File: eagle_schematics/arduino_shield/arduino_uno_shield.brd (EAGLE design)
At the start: 53 x 57.1 mm, 20 parts

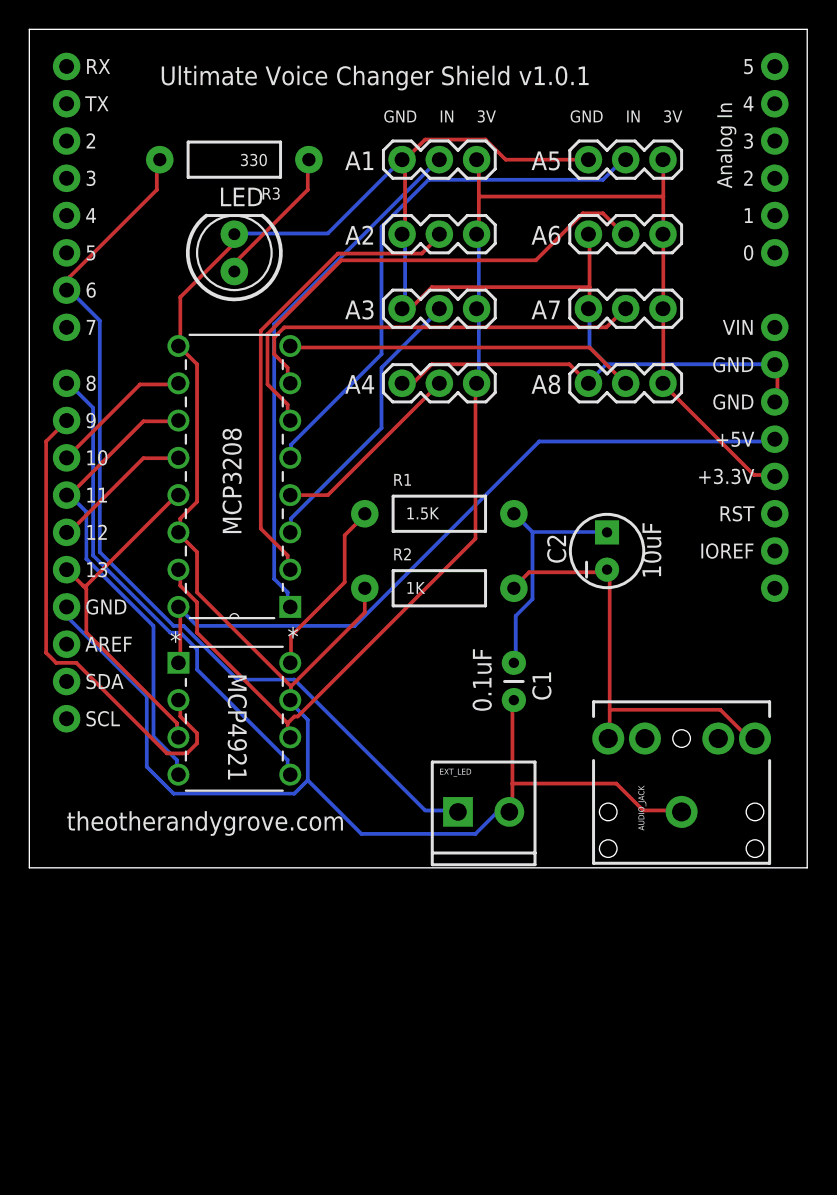
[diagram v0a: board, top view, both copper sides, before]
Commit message: save
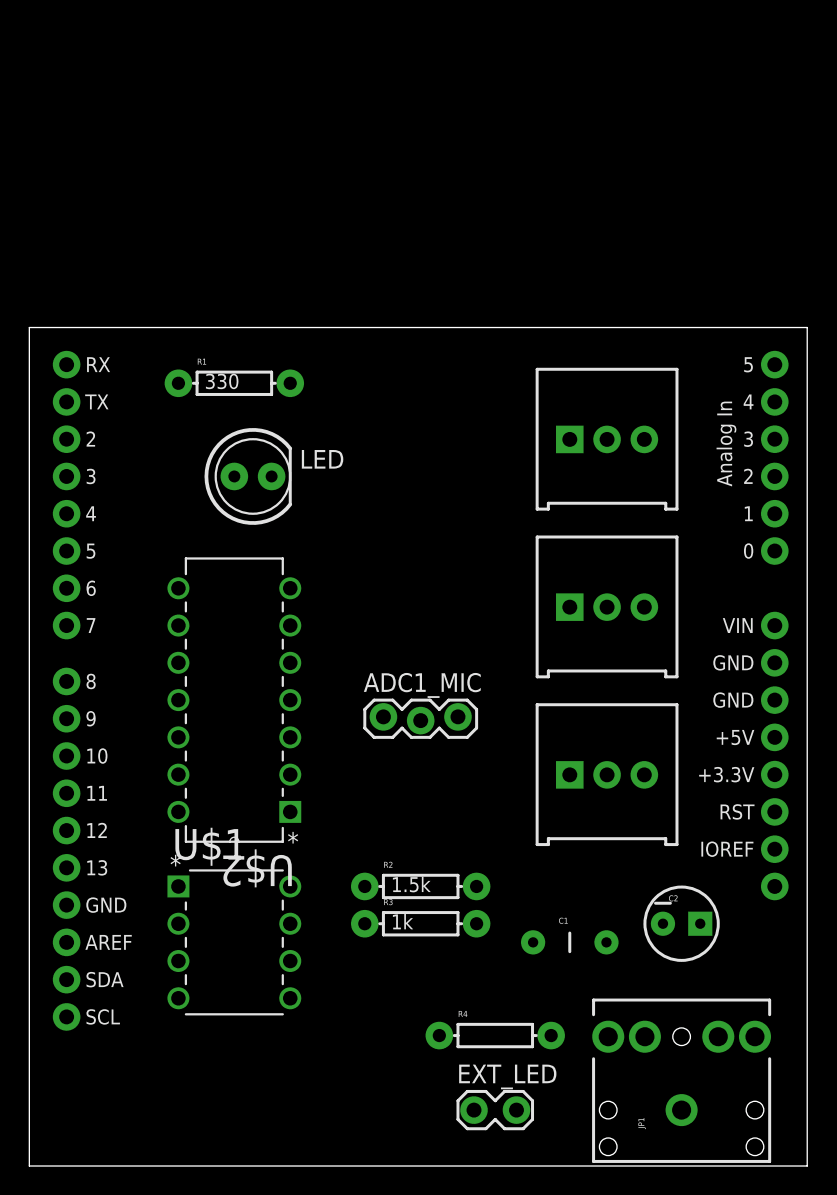
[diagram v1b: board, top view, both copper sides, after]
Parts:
- removed A1, A2, A3, A4, A5, A6, A7, A8: (no value), SparkFun-Connectors:1X03
- removed AUDIO_JACK: (no value), SparkFun-Connectors:AUDIO-JACK
- removed FRAME3: FRAME-LETTER, SparkFun-Aesthetics:CREATIVE_COMMONS
- removed MCP3208: MCP3208-CI/P, Microchip_By_element14_Batch_1:DIP254P762X432-16
- removed MCP4921: MCP4921-E/P, Microchip_By_element14_Batch_1:DIP254P762X432-8
- added ADC1_MIC: (no value), SparkFun-Connectors:1X03_LOCK
- added ADC2, ADC3, ADC4: TRIMPOT-PTH-KNOB, SparkFun-Electromechanical:3386U
- added JP1: (no value), SparkFun-Connectors:AUDIO-JACK
- added R4: (no value), SparkFun-Resistors:AXIAL-0.3
- added U$2: MCP3204-CI/P, Microchip_By_element14_Batch_1:DIP254P762X432-14
- added U1: ARDUINO_R3_SHIELD, SparkFun-Boards:UNO_R3_SHIELD
- C1: device SparkFun-Passives:CAP-PTH-SMALL -> SparkFun-Capacitors:CAP-PTH-5MM
- C2: device SparkFun-Passives:CPOL-RADIAL-10UF-25V -> SparkFun-Capacitors:CPOL-RADIAL-10UF-25V
- EXT_LED: value M023.5MM -> M02LOCK; device SparkFun-Connectors:SCREWTERMINAL-3.5MM-2 -> SparkFun-Connectors:1X02_LOCK
- R1: value 1.5K -> 330; device SparkFun-Passives:AXIAL-0.4 -> SparkFun-Resistors:AXIAL-0.3
- R2: value 1K -> 1.5k; device SparkFun-Passives:AXIAL-0.4 -> SparkFun-Resistors:AXIAL-0.3
- R3: value 330 -> 1k; device SparkFun-Passives:AXIAL-0.4 -> SparkFun-Resistors:AXIAL-0.3
- U$1: value ARDUINO_R3_SHIELD -> MCP4921-E/P; device SparkFun-Boards:UNO_R3_SHIELD -> Microchip_By_element14_Batch_1:DIP254P762X432-8
- moved R3 53.6 mm to (26.7, 16.5), turned to 0 degrees
- moved C2 25.9 mm to (44.5, 16.5), turned to 0 degrees
- moved EXT_LED 20.4 mm to (30.5, 3.81)
- moved R2 20.4 mm to (26.7, 19.1)
- moved U$1 19.9 mm to (17.8, 11.4)
- moved C1 19.4 mm to (36.8, 15.2), turned to 0 degrees
- moved R1 16.6 mm to (14.0, 53.3)
- moved LED 15.3 mm to (15.2, 47.0), turned to 0 degrees
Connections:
- removed net AUD: A1.2, MCP3208.1
- removed net N$10: LED.A, R3.P$1
- removed net N$11: MCP4921.5, U$1.D8
- removed net N$12: EXT_LED.1, R3.P$2, U$1.D6
- removed net N$14: A3.2, MCP3208.3
- removed net N$15: A4.2, MCP3208.4
- removed net N$16: A6.2, MCP3208.6
- removed net N$17: A7.2, MCP3208.7
- removed net N$18: A8.2, MCP3208.8
- removed net N$8: C1.1, C2.1, R1.P$2
- removed net N$9: AUDIO_JACK.RING, AUDIO_JACK.TIP, C2.2, R2.P$2
- removed net SPI_CLK: MCP3208.13, MCP4921.3, U$1.D13
- removed net SPI_MISO: MCP3208.12, U$1.D12
- removed net SPI_MOSI: MCP3208.11, MCP4921.4, U$1.D11
- new net ADC1: ADC1_MIC.1, U$2.1
- new net ADC2: ADC2.2, U$2.2
- new net ADC3: ADC3.2, U$2.3
- new net ADC4: ADC4.2, U$2.4
- new net LDAC: U$1.5, U1.D8
- new net LED: R1.P$1, R4.P$1, U1.D6
- new net MISO: U$2.10, U1.D12
- new net MOSI: U$1.4, U$2.9, U1.D11
- new net N$4: C2.2, JP1.RING, JP1.TIP, R3.P$2
- new net N$5: EXT_LED.1, R4.P$2
- new net SCK: U$1.3, U$2.11, U1.D13
- net 3.3V: now also ADC1_MIC.3, ADC2.1, ADC3.1, ADC4.1, U$1.6, U$2.13, U1.3.3V; no longer A1.3, A2.3, A3.3, A4.3, A5.3, A6.3, A7.3, A8.3, MCP3208.15, MCP4921.6, U$1.3.3V
- net 5V: now also U$1.1, U$2.14, U1.5V; no longer MCP3208.16, MCP4921.1, U$1.5V
- net CS_ADC: now also U$2.8, U1.D10; no longer MCP3208.10, U$1.D10
- net CS_DAC: now also U$1.2, U1.D9; no longer MCP4921.2, U$1.D9
- net GND: now also ADC1_MIC.2, ADC2.3, ADC3.3, ADC4.3, JP1.SLEEVE, R3.P$1, U$1.7, U$2.12, U$2.7, U1.GND@0; no longer A1.1, A2.1, A3.1, A4.1, A5.1, A6.1, A7.1, A8.1, AUDIO_JACK.SLEEVE, MCP3208.14, MCP3208.9, MCP4921.7, R2.P$1, U$1.GND@0, U$1.GND@1, U$1.GND@2
- net N$1: now also LED.A, R1.P$2; no longer A5.2, MCP3208.5
- net N$2: now also R2.P$1, U$1.8; no longer A2.2, MCP3208.2
- net N$3: now also C1.1, C2.1, R2.P$2; no longer MCP4921.8, R1.P$1
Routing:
- net GND: track 204.1 -> 0.00 mm
- net 3.3V: track 97.2 -> 0.00 mm
- net N$12: track 62.3 -> 0.00 mm
- net 5V: track 50.5 -> 0.00 mm
- net N$1: track 36.8 -> 0.00 mm
- net AUD: track 35.7 -> 0.00 mm
- net N$16: track 34.9 -> 0.00 mm
- net N$11: track 33.5 -> 0.00 mm
- net CS_DAC: track 33.3 -> 0.00 mm
- net N$2: track 32.1 -> 0.00 mm
- net SPI_MOSI: track 32.0 -> 0.00 mm
- net N$9: track 29.3 -> 0.00 mm
- net N$17: track 28.3 -> 0.00 mm
- net N$18: track 23.9 -> 0.00 mm
- net SPI_CLK: track 23.7 -> 0.00 mm
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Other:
- board text removed: "3V"
- board text removed: "GND"
- board text removed: "IN"
- board text removed: "Ultimate Voice Changer Shield v1.0.1"
- board text removed: "theotherandygrove.com"

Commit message: save
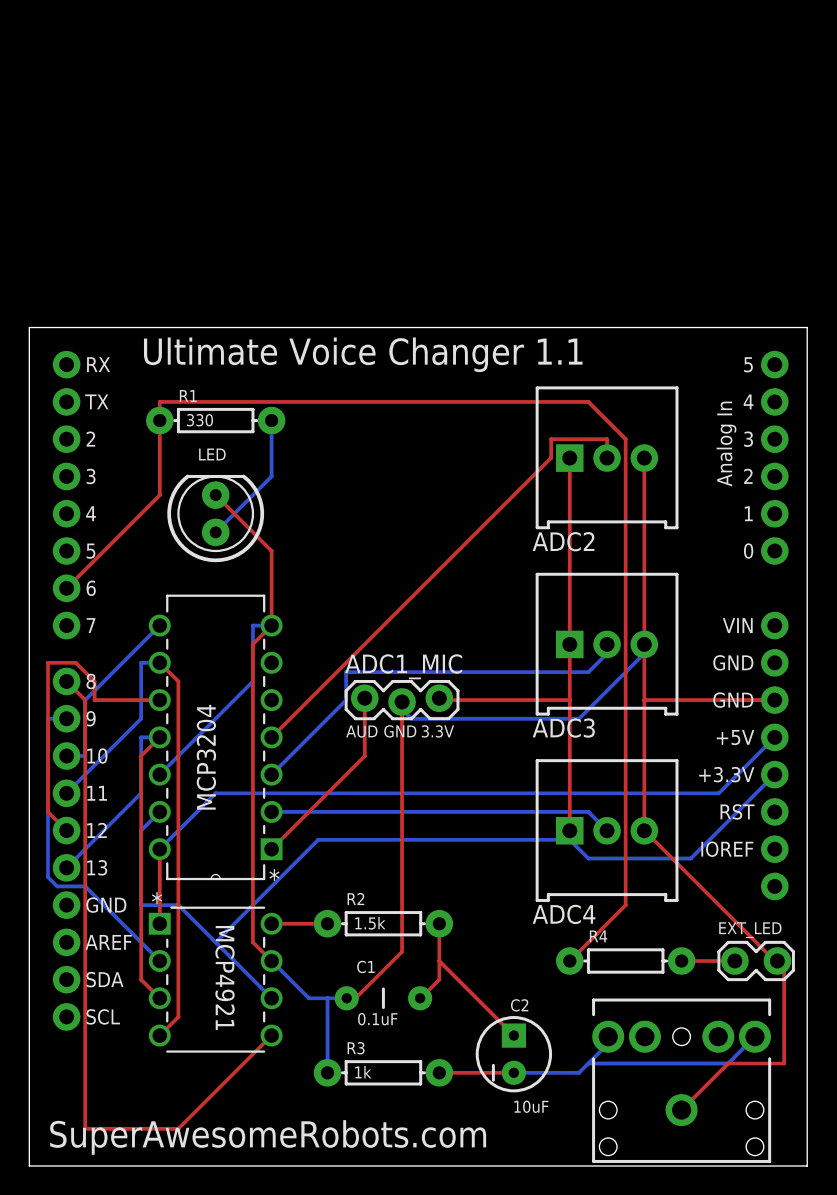
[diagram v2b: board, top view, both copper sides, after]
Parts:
- moved EXT_LED 20.5 mm to (48.3, 14.0)
- moved C2 14.5 mm to (33.0, 7.62), turned to 90 degrees
- moved C1 13.3 mm to (24.1, 11.4), turned to 180 degrees
- moved R3 10.5 mm to (24.1, 6.35)
- moved R4 10.2 mm to (40.6, 14.0)
- moved ADC2 3.81 mm to (39.4, 22.9)
- moved R2 3.59 mm to (24.1, 16.5)
- moved LED 3.59 mm to (12.7, 44.5), turned to 90 degrees
- moved R1 2.84 mm to (12.7, 50.8)
- moved U$1 2.84 mm to (16.5, 8.89)
- moved U$2 2.84 mm to (8.89, 36.8)
- moved ADC3 2.54 mm to (39.4, 35.6)
- moved ADC1_MIC 1.80 mm to (22.9, 31.8)
- moved ADC4 1.27 mm to (39.4, 48.3)
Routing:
- net GND: track 0.00 -> 164.3 mm
- net 3.3V: track 0.00 -> 97.3 mm
- net LED: track 0.00 -> 85.3 mm
- net 5V: track 0.00 -> 50.1 mm
- net LDAC: track 0.00 -> 46.3 mm
- net MOSI: track 0.00 -> 38.7 mm
- net ADC4: track 0.00 -> 33.3 mm
- net SCK: track 0.00 -> 31.1 mm
- net ADC3: track 0.00 -> 28.0 mm
- net N$4: track 0.00 -> 24.9 mm
- net ADC2: track 0.00 -> 23.4 mm
- net CS_DAC: track 0.00 -> 22.1 mm
- net MISO: track 0.00 -> 21.4 mm
- net ADC1: track 0.00 -> 12.9 mm
- net N$3: track 0.00 -> 12.8 mm
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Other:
- board text added: "3.3V"
- board text added: "ADC2"
- board text added: "ADC3"
- board text added: "ADC4"
- board text added: "AUD"
- board text added: "GND"
- board text added: "MCP3204"
- board text added: "MCP4921"
- board text added: "SuperAwesomeRobots.com"
- board text added: "Ultimate Voice Changer 1.1"
